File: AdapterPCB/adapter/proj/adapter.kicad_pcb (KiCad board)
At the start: 2 copper layers, 76.2 x 75.7 mm, 37 parts, among them J2 VGA, U1 SN74LVC245APW, U2 SN74LVC245APW

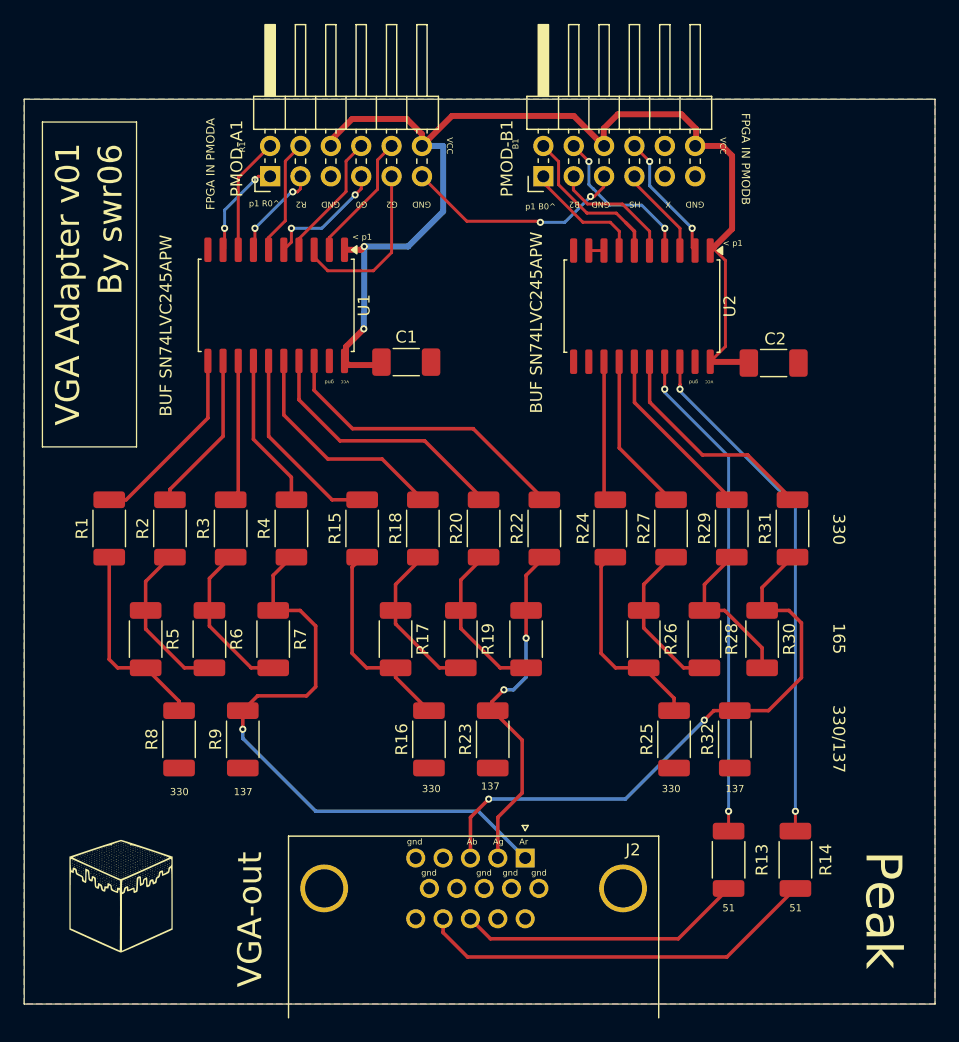
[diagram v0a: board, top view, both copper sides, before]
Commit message: fixed drc
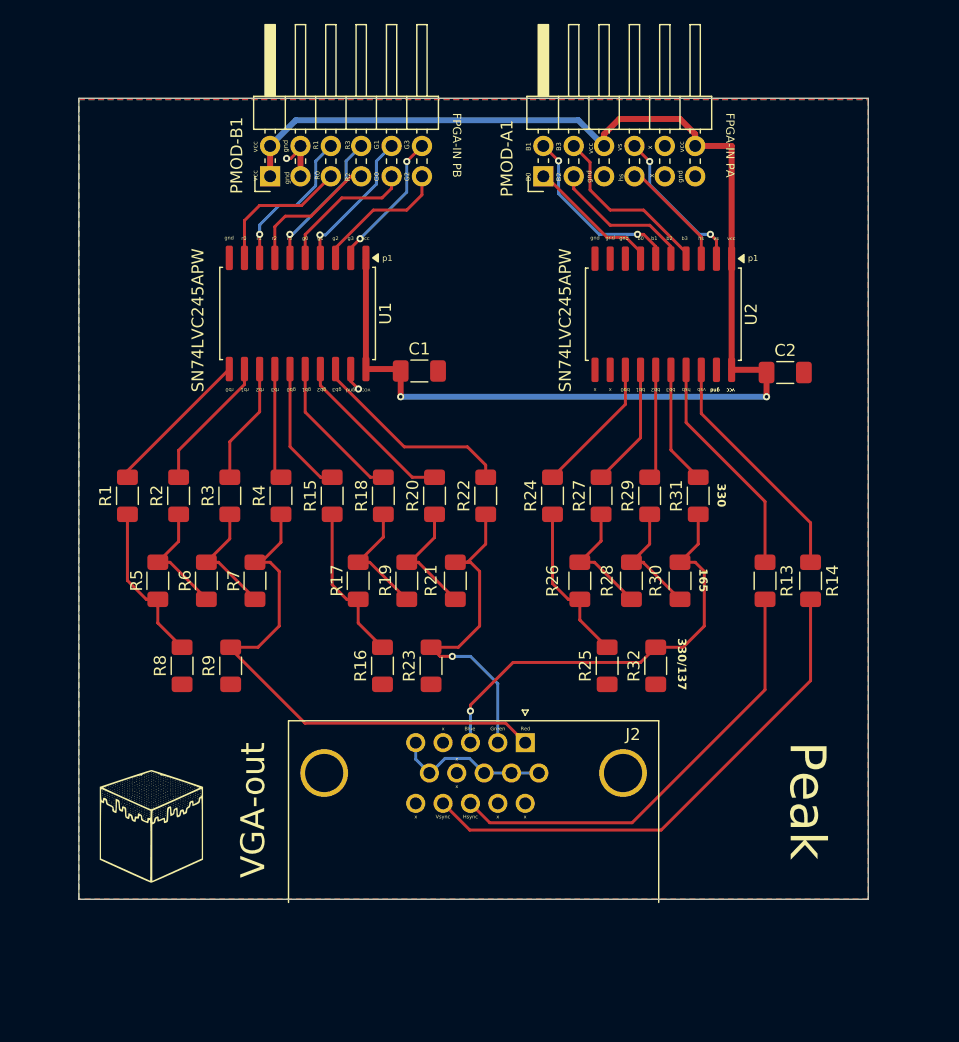
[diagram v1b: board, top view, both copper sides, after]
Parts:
- C1, C2: footprint Capacitor_SMD:C_1808_4520Metric -> Capacitor_SMD:C_1206_3216Metric_Pad1.33x1.80mm_HandSolder
- R1, R13, R14, R15, R16, R17, R18, R19, R2, R20, R21, R22, R23, R24, R25, R26, R27, R28, R29, R3, R30, R31, R32, R4, R5, R6, R7, R8, R9: footprint Resistor_SMD:R_2010_5025Metric_Pad1.40x2.65mm_HandSolder -> Resistor_SMD:R_1206_3216Metric_Pad1.30x1.75mm_HandSolder
- moved R13 23.5 mm to (169.2, 85.9)
- moved R14 23.4 mm to (173.0, 85.9)
- moved J2 9.65 mm to (149.1, 99.4)
- moved R32 9.03 mm to (160.0, 93.0)
- moved R30 8.43 mm to (162.1, 85.9)
- moved R31 8.34 mm to (163.6, 78.8)
- moved R25 8.32 mm to (156.0, 93.0)
- moved R23 8.03 mm to (141.2, 93.0)
- moved R28 7.82 mm to (158.0, 85.9)
- moved R21 7.67 mm to (143.3, 85.9)
- moved R29 7.39 mm to (159.5, 78.8)
- moved R16 7.28 mm to (137.2, 93.0)
- moved R26 7.24 mm to (153.7, 85.9)
- moved R19 6.65 mm to (139.2, 85.9)
- moved R27 6.46 mm to (155.4, 78.8)
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- renumbered PMOD-B1 to PMOD-A1, PMOD-A1 to PMOD-B1
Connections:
- PMOD-B1 pad 1: R0 -> VCC33
- PMOD-B1 pad 10: G3 -> G1
- PMOD-B1 pad 11: GND -> G2
- PMOD-B1 pad 12: VCC33 -> G3
- PMOD-B1 pad 2: R1 -> VCC33
- PMOD-B1 pad 3: R2 -> GND
- PMOD-B1 pad 4: R3 -> GND
- PMOD-B1 pad 5: GND -> R0
- PMOD-B1 pad 6: VCC33 -> R1
- PMOD-B1 pad 7: G0 -> R2
- PMOD-B1 pad 8: G1 -> R3
- PMOD-B1 pad 9: G2 -> G0
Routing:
- net VSyncb: track 43.3 -> 19.9 mm, vias 2 -> 0
- net HSyncb: track 41.5 -> 18.8 mm, vias 2 -> 0
- net VCC33: track 95.6 -> 115.1 mm
- net Net-(J2-Pad13): track 24.0 -> 37.5 mm
- net AnalogB: track 49.7 -> 37.0 mm, vias 2 -> 1
- net Net-(J2-Pad14): track 33.8 -> 43.7 mm
- net Bb3: track 18.7 -> 9.93 mm
- net Gb3: track 25.5 -> 17.4 mm
- net Gb2: track 22.2 -> 14.1 mm
- net Gb1: track 19.1 -> 12.4 mm
- net AnalogR: track 51.3 -> 45.5 mm, vias 1 -> 0
- net Bb2: track 14.9 -> 9.20 mm
- net Gb0: track 16.3 -> 11.1 mm
- net Net-(R15-Pad1): track 17.3 -> 13.4 mm
- net R0: track 8.35 -> 12.1 mm, vias 2 -> 0
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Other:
- board size 76.2 x 75.7 mm -> 66 x 67 mm
- board text added: "B0"
- board text added: "B3"
- board text added: "Blue"
- board text added: "FPGA-IN PA"
- board text added: "FPGA-IN PB"
- board text added: "G1"
- board text added: "G3"
- board text added: "Green"
- board text added: "Hsync"
- board text added: "R0"
- board text added: "R3"
- board text added: "Red"
- board text added: "SN74LVC245APW"
- board text added: "Vsync"
- board text added: "b0"
- board text added: "b1"
- board text added: "b2"
- board text added: "b3"
- board text added: "bb0"
- board text added: "bb1"
- board text added: "bb2"
- board text added: "bb3"
- board text added: "g0"
- board text added: "g1"
- board text added: "g2"
- board text added: "g3"
- board text added: "gb0"
- board text added: "gb1"
- board text added: "gb2"
- board text added: "gb3"
- board text added: "hs"
- board text added: "hsb"
- board text added: "r0"
- board text added: "r1"
- board text added: "r2"
- board text added: "r3"
- board text added: "rb0"
- board text added: "rb1"
- board text added: "rb2"
- board text added: "rb3"
- board text added: "vs"
- board text added: "vsb"
- board text added: "x"
- board text removed: "137"
- board text removed: "51"
- board text removed: "Ab"
- board text removed: "Ag"
- board text removed: "Ar"
- board text removed: "BUF SN74LVC245APW"
- board text removed: "By swr06"
- board text removed: "FPGA IN PMODA"
- board text removed: "FPGA IN PMODB"
- board text removed: "GND"
- board text removed: "HS"
- board text removed: "VCC"
- board text removed: "VGA Adapter v01"
- board text removed: "X"
- board text removed: "p1 B0^"
- board text removed: "p1 R0^"
